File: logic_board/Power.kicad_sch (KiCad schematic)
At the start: 15 parts, among them J3 USB_C_Receptacle_USB2.0_16P, J5 Conn_01x02, SW5 SW_SPDT, U3 MCP73832-2-OT, U4 AP2112K-3.3, U5 USBLC6-2SC6

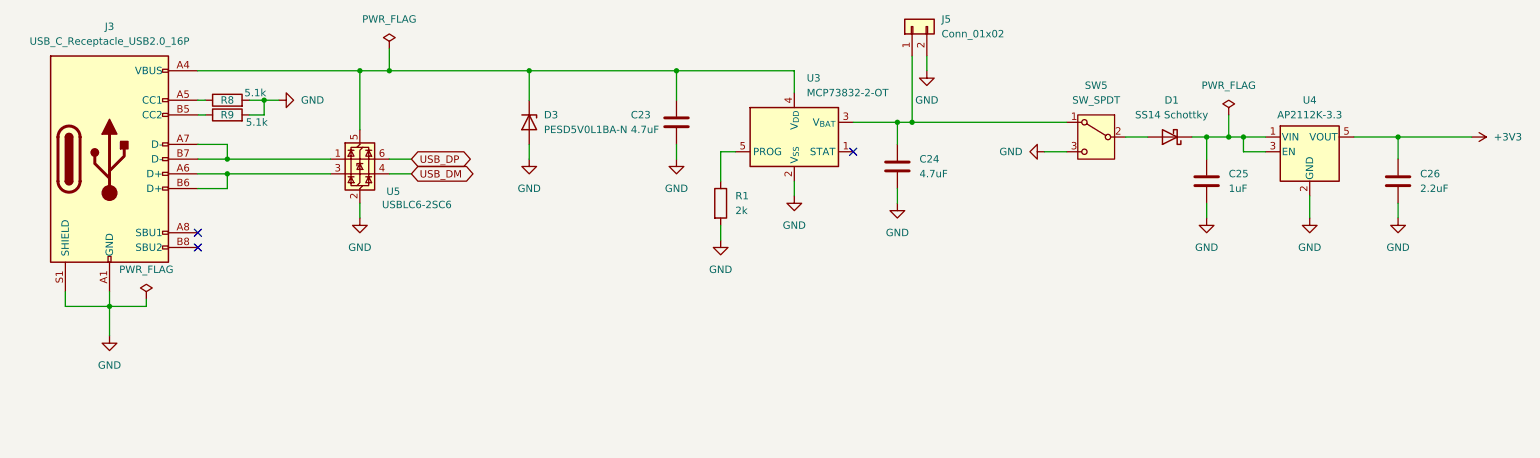
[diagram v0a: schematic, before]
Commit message: All signals now routed.
A bit rough, needs some cleanup.
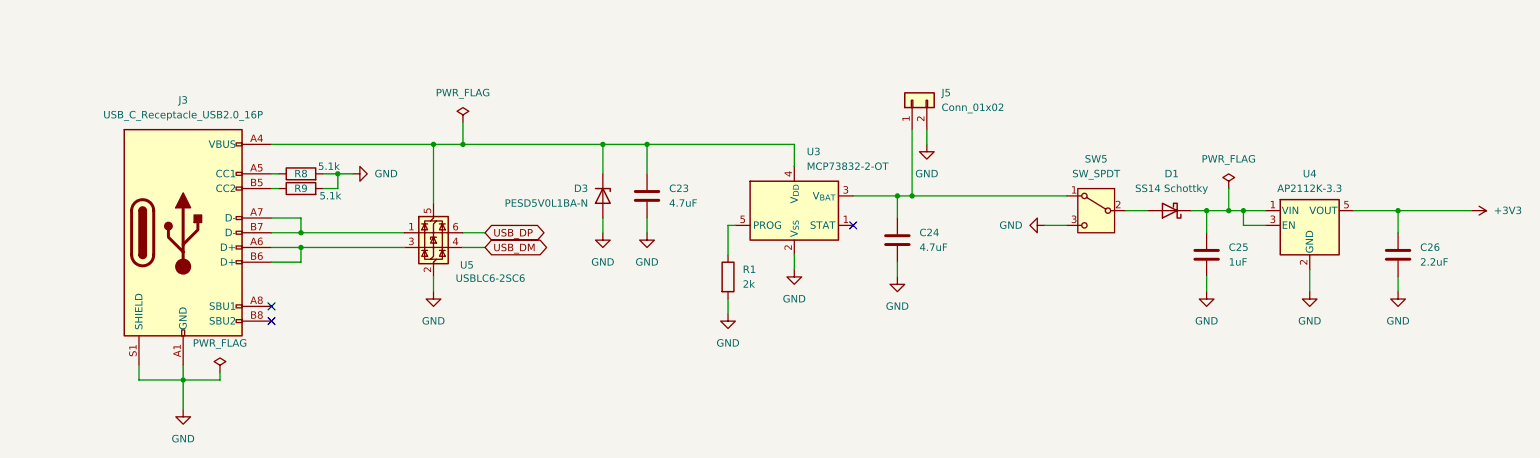
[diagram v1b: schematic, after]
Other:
- moved on the sheet: C23, C24, C25, C26, D1, D3, J3, J5, R1, R8, R9, SW5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
